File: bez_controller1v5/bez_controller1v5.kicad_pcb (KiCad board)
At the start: 4 copper layers, 75 parts, among them J1 Conn_01x03_Male, J10 IMU Conn_01x03_Female, J11 Conn_01x03_Male, J12 Conn_01x03_Male, J13 USB_B_Mini, J2 Conn_01x03_Male, J3 Conn_01x03_Male, J4 Screw_Terminal_01x02, J5 Conn_01x03_Male, J6 Conn_01x03_Male, J7 Conn_01x03_Male, J8 JTAG Conn_01x06_Male, J9 IMU Conn_01x08_Female, U1 PX07806-500-S, U10 USBLC6-4SC6, U11 74LVC2G241, U12 74LVC2G241, U2 74LVC2G241, U3 74LVC2G241, U4 LF50ABV_TO220, U5 LD1117AS33TR_SOT223, U6 INA180A1, U7 STM32F446RETx, U8 74LVC2G241, U9 74LVC2G241, Y1 8MHz

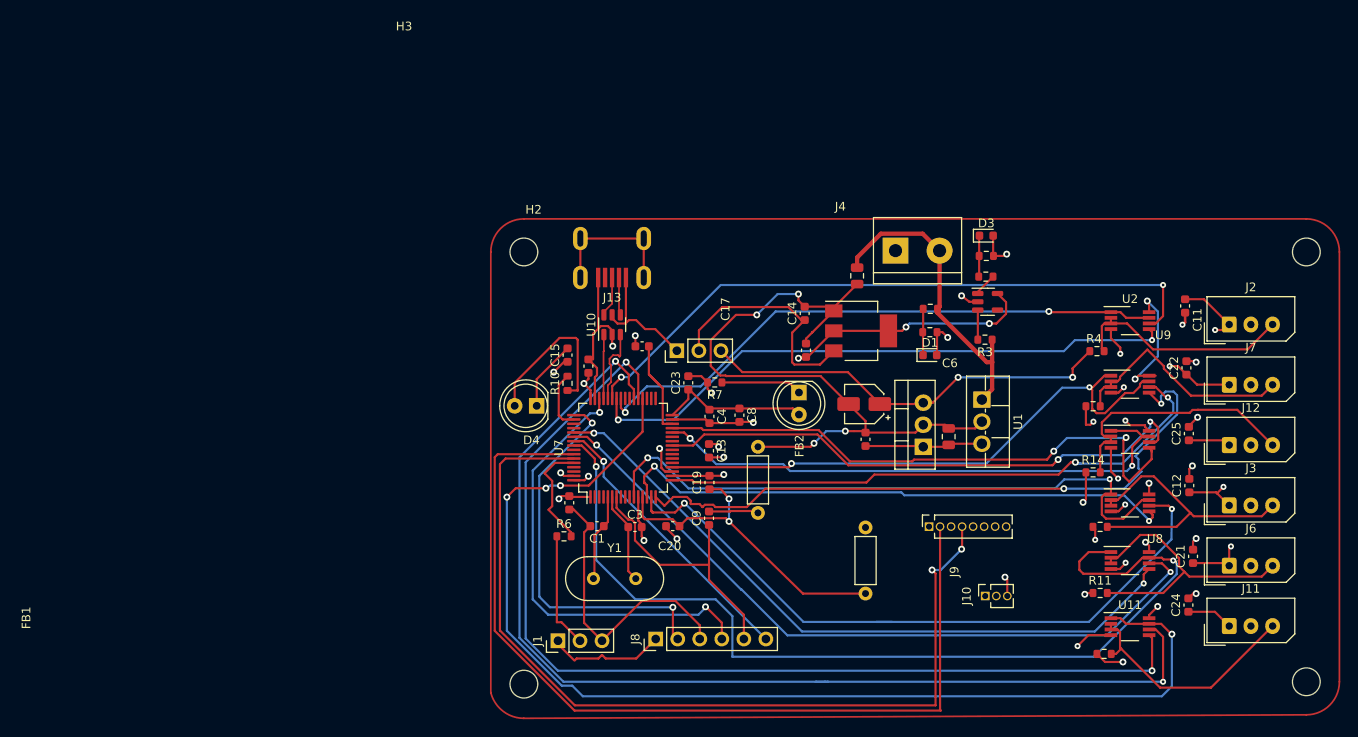
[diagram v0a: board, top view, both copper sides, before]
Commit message: new route PCB
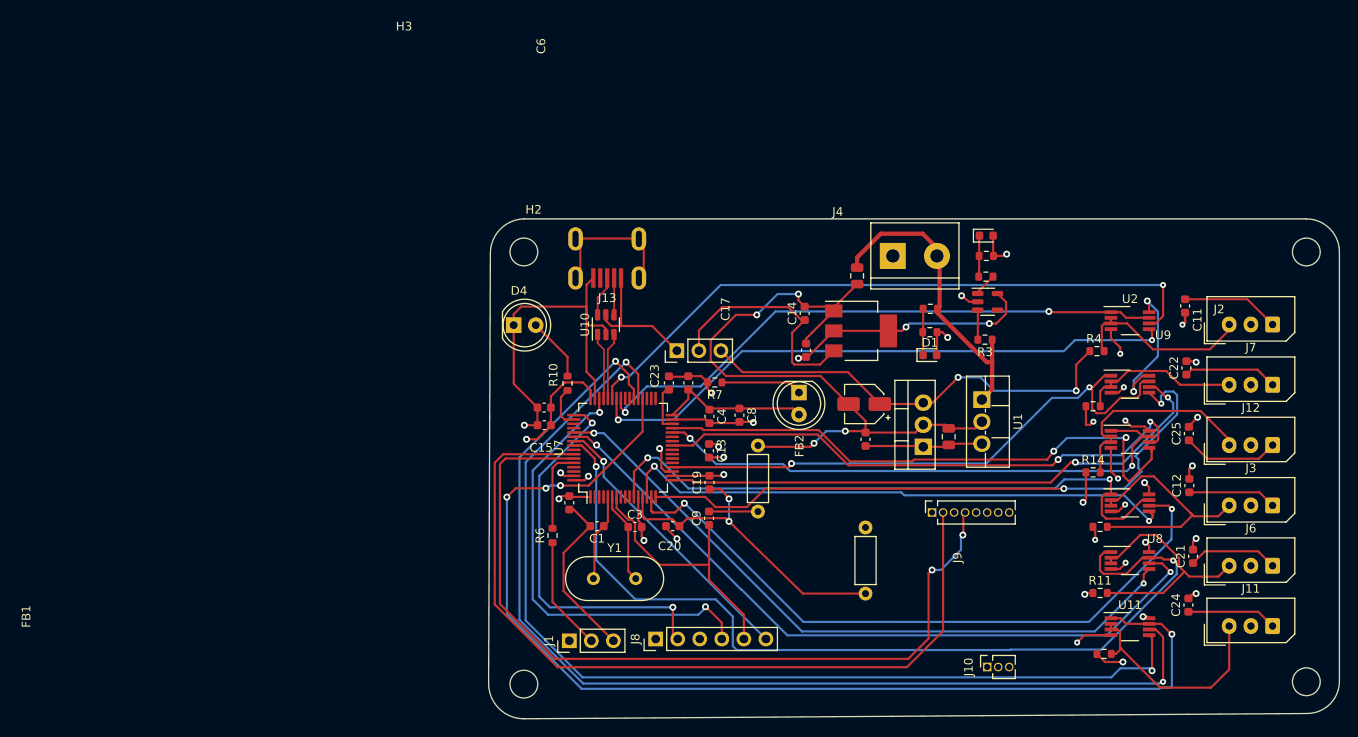
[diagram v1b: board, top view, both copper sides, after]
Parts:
- moved D4 9.67 mm to (34.4, 40.2), turned to 0 degrees
- moved C15 8.51 mm to (37.9, 51.7), turned to 180 degrees
- moved J10 8.18 mm to (89.0, 79.6)
- moved C6 6.99 mm to (37.9, 49.7), turned to 180 degrees
- moved C16 5.24 mm to (52.3, 46.9), turned to 90 degrees
- moved J9 1.66 mm to (82.6, 61.8)
- moved R6 1.32 mm to (38.9, 64.4), turned to 90 degrees
- moved J1 1.31 mm to (40.8, 76.6)
- moved U10 0.72 mm to (45.0, 40.1)
- moved J4 0.68 mm to (78.1, 32.2)
- moved J13 0.56 mm to (45.2, 28.3)
- moved FB1 0.15 mm to (62.5, 61.7)
- turned R10 to -90 degrees
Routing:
- net GND: track 179.9 -> 194.4 mm, vias 23 -> 17
- net Net-(D4-A): track 19.2 -> 7.40 mm
- net /I2C_SDA: track 104.9 -> 95.0 mm
- net /I2C_SCL: track 105.7 -> 95.9 mm
- net /MOTOR_DATA2: track 27.0 -> 18.6 mm
- net Net-(U7-VCAP_1): track 12.4 -> 5.48 mm
- net +3.3V: track 76.9 -> 70.9 mm, vias 9 -> 8
- net /USART5_DIR: track 112.2 -> 106.4 mm
- net /MOTOR_DATA1: track 25.9 -> 20.4 mm
- net /MOTOR_DATA5: track 33.3 -> 28.8 mm
- net /MOTOR_DATA4: track 33.1 -> 28.9 mm
- net /MOTOR_DATA3: track 29.6 -> 25.4 mm
- net +5V: track 83.5 -> 87.1 mm
- net /BOOT0: track 12.8 -> 9.66 mm
- net /USART6_RX: track 126.7 -> 124.0 mm
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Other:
- board outline added: 98 x 57.6 mm
